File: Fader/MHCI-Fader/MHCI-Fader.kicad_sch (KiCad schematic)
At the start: 11 parts, among them J1 RJ12, SW1 SW_Push_LED, U1 ISOW1044

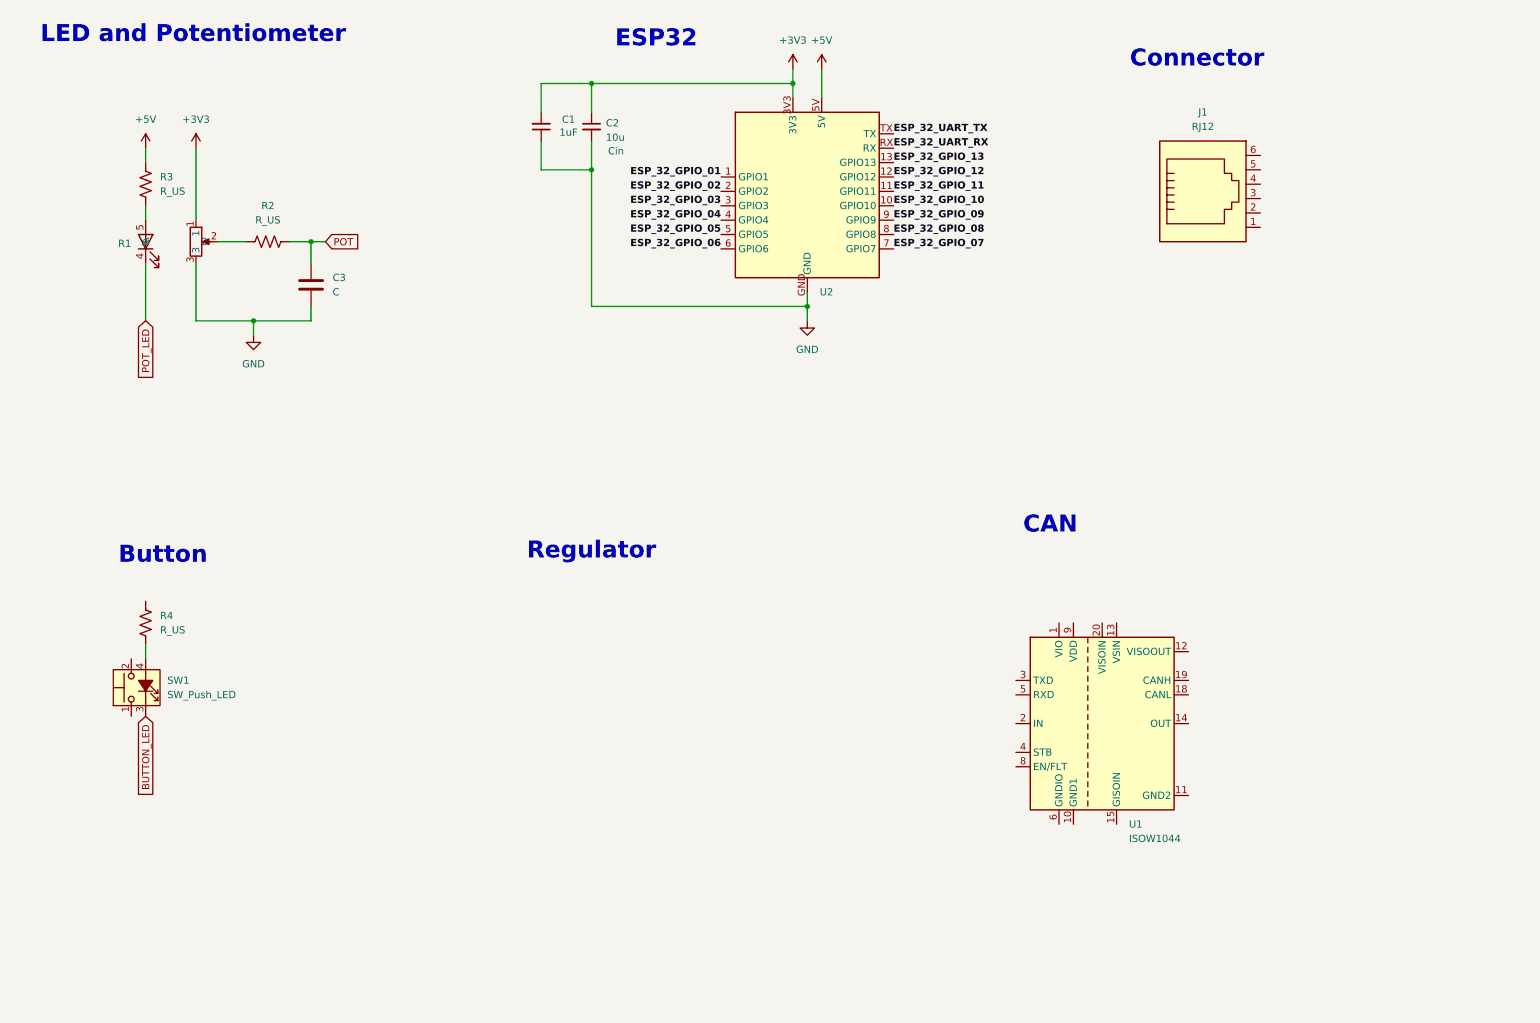
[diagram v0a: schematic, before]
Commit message: Initial fader schematic
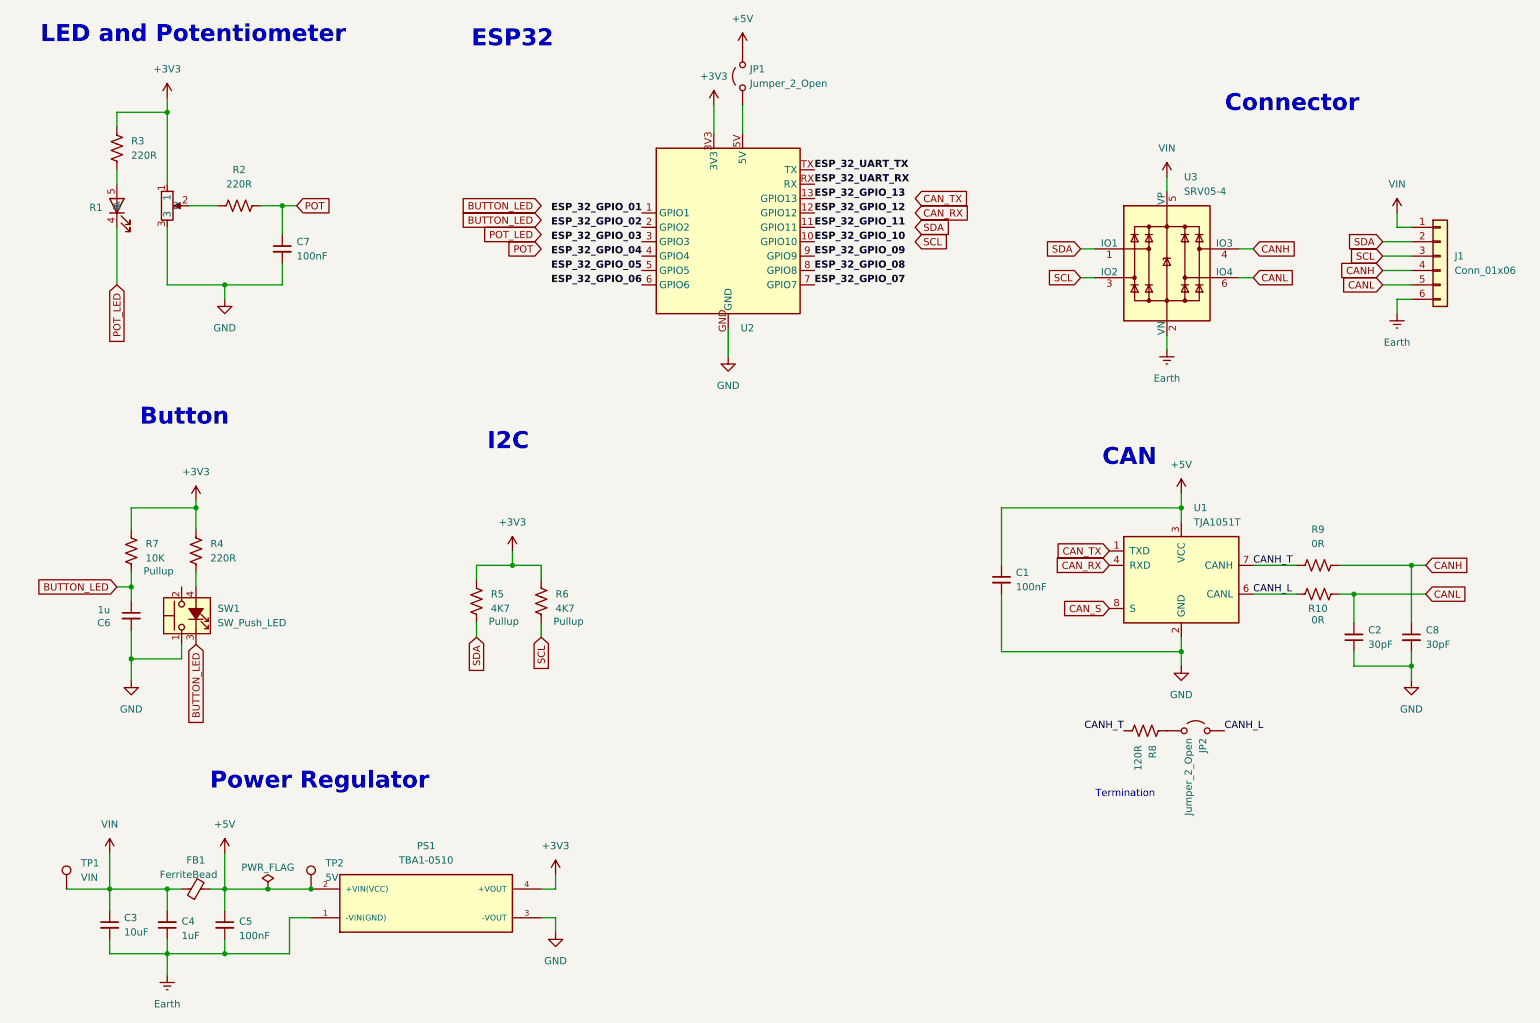
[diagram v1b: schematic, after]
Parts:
- removed C3: C, symbol Device:C
- removed J1: RJ12, Connector_RJ:RJ12_Amphenol_54601-x06_Horizontal, symbol Connector:RJ12
- removed U1: ISOW1044, Package_SO:SOIC-20W_7.5x12.8mm_P1.27mm, symbol Interface_CAN_LIN:ISOW1044
- added C3: 10uF, Capacitor_SMD:C_0603_1608Metric, symbol Device:C_Small
- added C4: 1uF, Capacitor_SMD:C_0402_1005Metric, symbol Device:C_Small
- added C5, C7: 100nF, Capacitor_SMD:C_0402_1005Metric, symbol Device:C_Small
- added C6: 1u, Capacitor_SMD:C_0402_1005Metric, symbol Device:C_Small
- added C8: 30pF, Capacitor_SMD:C_0402_1005Metric, symbol Device:C_Small
- added FB1: FerriteBead, Diode_SMD:D_0805_2012Metric, symbol Device:FerriteBead_Small
- added J1: Conn_01x06, Connector_PinHeader_2.54mm:PinHeader_1x06_P2.54mm_Vertical, symbol Connector_Generic:Conn_01x06
- added JP1, JP2: Jumper_2_Open, Jumper:SolderJumper-2_P1.3mm_Open_RoundedPad1.0x1.5mm, symbol Jumper:Jumper_2_Open
- added PS1: TBA1-0510, MCHI:CONV_TBA1-0510, symbol MHCI:TBA1-0510
- added R10, R9: 0R, Resistor_SMD:R_0402_1005Metric, symbol Device:R_US
- added R5, R6: 4K7, Resistor_SMD:R_0603_1608Metric, symbol Device:R_US
- added R7: 10K, Resistor_SMD:R_0402_1005Metric, symbol Device:R_US
- added R8: 120R, Resistor_SMD:R_0402_1005Metric, symbol Device:R_US
- added TP1: VIN, TestPoint:TestPoint_Pad_D1.0mm, symbol Connector:TestPoint
- added TP2: 5V, TestPoint:TestPoint_Pad_D1.0mm, symbol Connector:TestPoint
- added U1: TJA1051T, Package_SO:SOIC-8_3.9x4.9mm_P1.27mm, symbol Interface_CAN_LIN:TJA1051T
- added U3: SRV05-4, Package_TO_SOT_SMD:SOT-23-6, symbol Power_Protection:SRV05-4
- C1: value 1uF -> 100nF; LCSC C52923 -> C1525
- C2: value 10u -> 30pF; footprint Capacitor_SMD:C_0603_1608Metric -> Capacitor_SMD:C_0402_1005Metric; LCSC C19702 -> C1570
- R2, R3, R4: value R_US -> 220R; footprint (none) -> Resistor_SMD:R_0402_1005Metric; LCSC (none) -> C25091
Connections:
- net +3V3: now also R3.2, R4.2, PS1.4 (+VOUT), R5.1, R6.1, R7.1; no longer C1.2, C2.1
- net +5V: now also C1.1, C5.1, FB1.2, JP1.2 (B), PS1.2 (+VIN(VCC)), TP2.1, U1.3 (VCC); no longer R3.2, U2.5V
- net BUTTON_LED: now also C6.1, R7.2
- net GND: now also C1.2, C2.1, SW1.1, C6.2, C7.2, C8.2, PS1.3 (-VOUT), U1.2 (GND); no longer C1.1, C2.2
- net POT: now also R2.1, C7.1; no longer R2.2
- net at R1.2: now also R2.2; no longer R2.1
- new net: JP2.1 (A), R8.2
- new net: JP1.1 (A), U2.5V
- new net CANH: C8.1, J1.4 (Pin_4), R9.1, U3.4 (IO3)
- new net CANH_L: JP2.2 (B), R10.1, U1.6 (CANL)
- new net CANH_T: R8.1, R9.2, U1.7 (CANH)
- new net CANL: C2.2, J1.5 (Pin_5), R10.2, U3.6 (IO4)
- new net CAN_RX: U1.4 (RXD)
- new net CAN_S: U1.8 (S)
- new net CAN_TX: U1.1 (TXD)
- new net Earth: C3.2, C4.1, C5.2, J1.6 (Pin_6), PS1.1 (-VIN(GND)), U3.2 (VN)
- new net SCL: J1.3 (Pin_3), R6.2, U3.3 (IO2)
- new net SDA: J1.2 (Pin_2), R5.2, U3.1 (IO1)
- new net VIN: C3.1, C4.2, FB1.1, J1.1 (Pin_1), TP1.1, U3.5 (VP)
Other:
- note added: "I2C"
- note added: "Power Regulator"
- note added: "Termination"
- note removed: "Regulator"
- moved on the sheet: R1, R3, SW1, U2
